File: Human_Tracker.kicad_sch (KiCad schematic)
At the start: 59 parts, among them U1 TPS54233QDRQ1, U2 ICS-43434_C5656610, U3 ICS-43434_C5656610, U4 ADM7172ACPZ-3.3-R7, U5 BME680, U6 ESP32-S3-WROOM-1(N16R8), U7 MLX90640ESF-BAB-000-TU, U8 FRC0805F1400TS 140

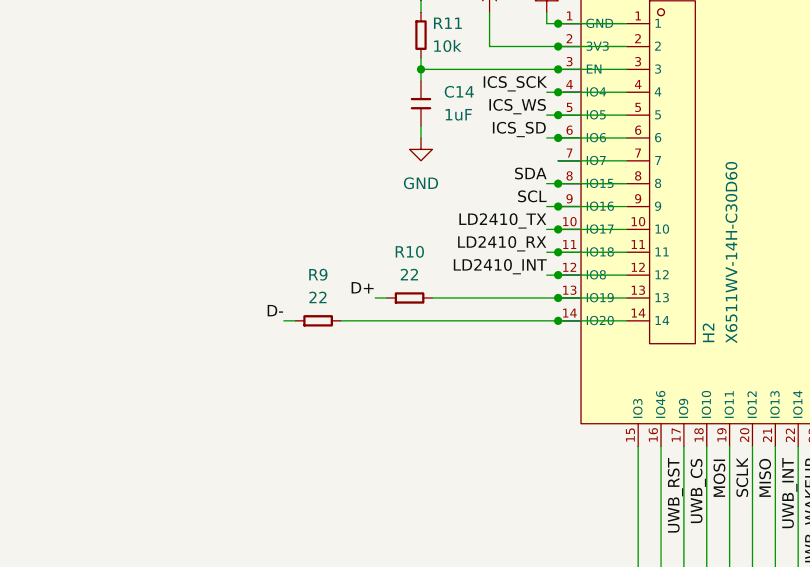
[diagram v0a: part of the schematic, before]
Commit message: layout amelioré V67
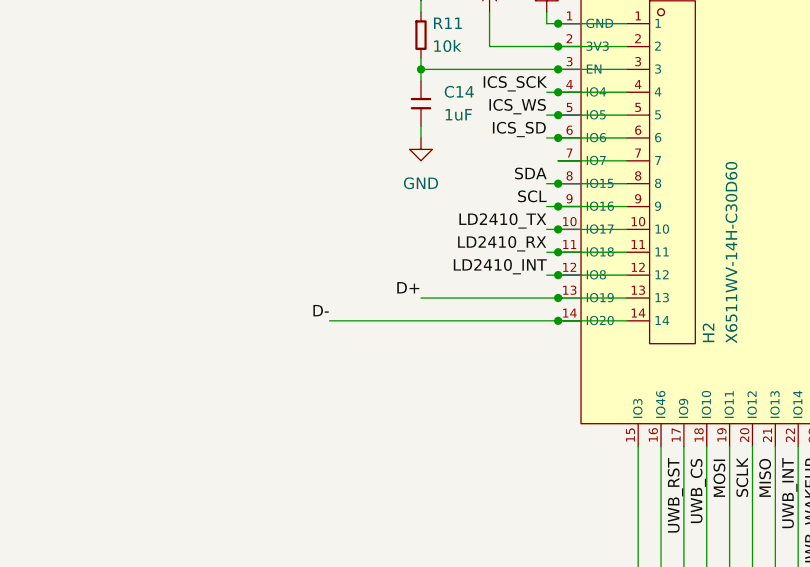
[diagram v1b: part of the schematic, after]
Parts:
- removed R10, R9: 22, lcsc_footprints:C17414_R0805, symbol Custom_Device:R
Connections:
- net D+: now also H2.13, U6.13 (IO19)
- net D-: now also H2.14, U6.14 (IO20)
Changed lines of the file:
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@@
 	(wire
 		(pts
-			(xy 252.73 222.25) (xy 254 222.25)
+			(xy 257.81 222.25) (xy 283.21 222.25)
 		)
 		(stroke
@@
 	(wire
 		(pts
-			(xy 259.08 222.25) (xy 283.21 222.25)
-		)
-		(stroke
-			(width 0)
-			(type default)
-		)
-	)
-	(wire
-		(pts
-			(xy 269.24 219.71) (xy 283.21 219.71)
-		)
-		(stroke
-			(width 0)
-			(type default)
-		)
-	)
-	(wire
-		(pts
 			(xy 302.26 80.01) (xy 302.26 87.63)
 		)
@@
 	(wire
 		(pts
-			(xy 262.89 219.71) (xy 264.16 219.71)
+			(xy 267.97 219.71) (xy 283.21 219.71)
 		)
 		(stroke
@@
 	)
 	(label "D-"
-		(at 252.73 222.25 180)
+		(at 257.81 222.25 180)
 		(effects
 			(font
@@
 	)
 	(label "D+"
-		(at 262.89 219.71 180)
+		(at 267.97 219.71 180)
 		(effects
 			(font
@@
 	)
 	(symbol
-		(lib_id "Custom_Device:R")
-		(at 266.7 219.71 90)
-		(unit 1)
-		(body_style 1)
-		(exclude_from_sim no)
-		(in_bom yes)
-		(on_board yes)
-		(in_pos_files yes)
-		(dnp no)
-		(fields_autoplaced yes)
-		(property "Reference" "R10"
-			(at 266.7 214.63 90)
-			(show_name no)
-			(do_not_autoplace no)
-			(effects
-				(font
-					(size 1.27 1.27)
-				)
-			)
-		)
-		(property "Value" "22"
-			(at 266.7 217.17 90)
-			(show_name no)
-			(do_not_autoplace no)
-			(effects
-				(font
-					(size 1.27 1.27)
-				)
-			)
-		)
-		(property "Footprint" "lcsc_footprints:C17414_R0805"
-			(at 266.7 221.488 90)
-			(hide yes)
-			(show_name no)
-			(do_not_autoplace no)
-			(effects
-				(font
-					(size 1.27 1.27)
-				)
-			)
-		)
-		(property "Datasheet" ""
-			(at 266.7 219.71 0)
-			(hide yes)
-			(show_name no)
-			(do_not_autoplace no)
-			(effects
-				(font
-					(size 1.27 1.27)
-				)
-			)
-		)
-		(property "Description" "Resistor"
-			(at 266.7 219.71 0)
-			(hide yes)
-			(show_name no)
-			(do_not_autoplace no)
-			(effects
-				(font
-					(size 1.27 1.27)
-				)
-			)
-		)
-		(property "LCSC" "C17561"
-			(at 266.7 219.71 90)
-			(hide yes)
-			(show_name no)
-			(do_not_autoplace no)
-			(effects
-				(font
-					(size 1.27 1.27)
-				)
-			)
-		)
-		(pin "2"
-		)
-		(pin "1"
-		)
-		(instances
-			(project "Human_Tracker"
-				(path "/21992c97-7c29-4ade-9a85-42ee1fb0a3a3"
-					(reference "R10")
-					(unit 1)
-				)
-			)
-		)
-	)
-	(symbol
 		(lib_id "Connector:TestPoint")
 		(at 419.1 233.68 180)
@@
 					(unit 1)
 				)
-			)
-		)
-	)
-	(symbol
-		(lib_id "Custom_Device:R")
-		(at 256.54 222.25 90)
-		(unit 1)
-		(body_style 1)
-		(exclude_from_sim no)
-		(in_bom yes)
-		(on_board yes)
-		(in_pos_files yes)
-		(dnp no)
-		(fields_autoplaced yes)
-		(property "Reference" "R9"
-			(at 256.54 217.17 90)
-			(show_name no)
-			(do_not_autoplace no)
-			(effects
-				(font
-					(size 1.27 1.27)
-				)
-			)
-		)
-		(property "Value" "22"
-			(at 256.54 219.71 90)
-			(show_name no)
-			(do_not_autoplace no)
-			(effects
-				(font
-					(size 1.27 1.27)
-				)
-			)
-		)
-		(property "Footprint" "lcsc_footprints:C17414_R0805"
-			(at 256.54 224.028 90)
-			(hide yes)
-			(show_name no)
-			(do_not_autoplace no)
-			(effects
-				(font
-					(size 1.27 1.27)
-				)
-			)
-		)
-		(property "Datasheet" ""
-			(at 256.54 222.25 0)
-			(hide yes)
-			(show_name no)
-			(do_not_autoplace no)
-			(effects
-				(font
-					(size 1.27 1.27)
-				)
-			)
-		)
-		(property "Description" "Resistor"
-			(at 256.54 222.25 0)
-			(hide yes)
-			(show_name no)
-			(do_not_autoplace no)
-			(effects
-				(font
-					(size 1.27 1.27)
-				)
-			)
-		)
-		(property "LCSC" "C17561"
-			(at 256.54 222.25 90)
-			(hide yes)
-			(show_name no)
-			(do_not_autoplace no)
-			(effects
-				(font
-					(size 1.27 1.27)
-				)
-			)
-		)
-		(pin "2"
-		)
-		(pin "1"
-		)
-		(instances
-			(project "Human_Tracker"
-				(path "/21992c97-7c29-4ade-9a85-42ee1fb0a3a3"
-					(reference "R9")
-					(unit 1)
-				)
